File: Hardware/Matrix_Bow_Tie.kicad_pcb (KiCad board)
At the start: 2 copper layers, 116.8 x 55.9 mm, 81 parts, among them J1 CONN_12, J2 CONN_12, Q1 TRANS_NPN_DUAL-MBT3904DW1T1, Q2 TRANS_NPN_DUAL-MBT3904DW1T1, Q3 TRANS_NPN_DUAL-MBT3904DW1T1, Q4 TRANS_NPN_DUAL-MBT3904DW1T1, U1 MAX4466, U2 74HC4051-SOIC16

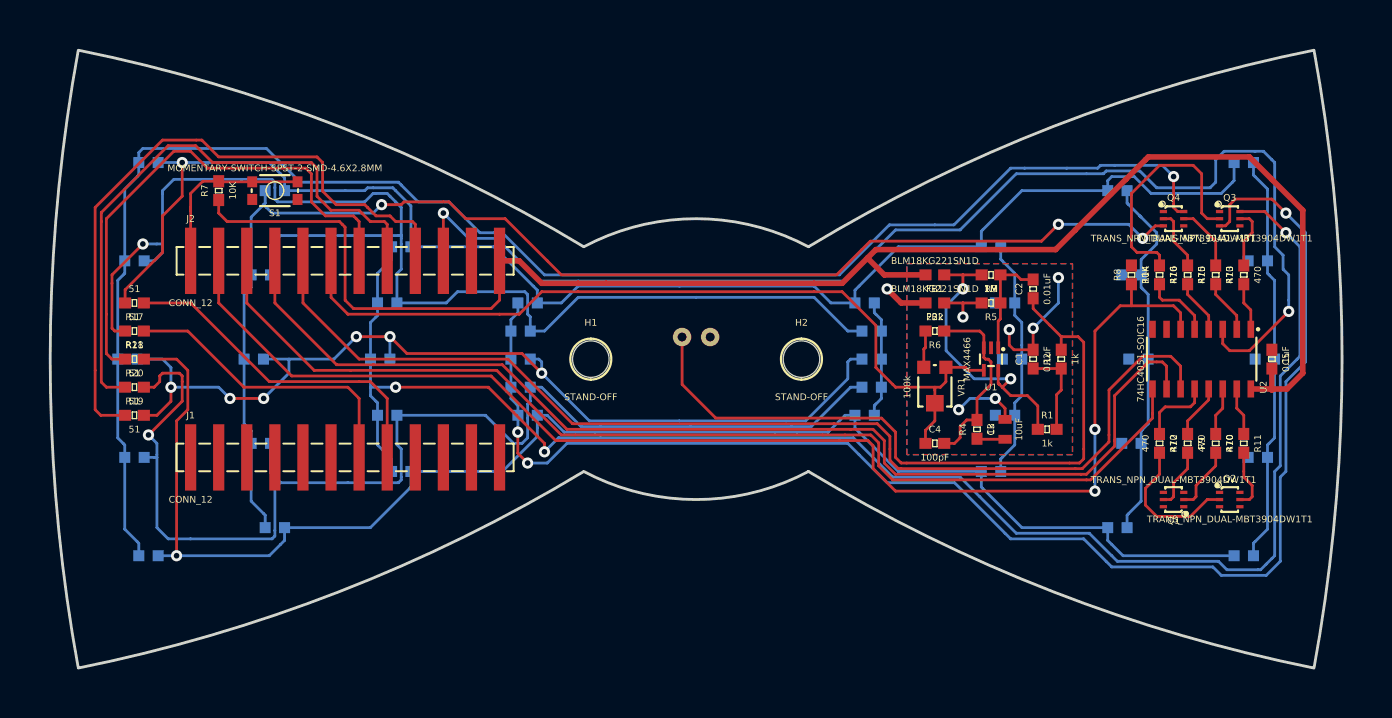
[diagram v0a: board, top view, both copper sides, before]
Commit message: Layout complete. Gerbers ran.
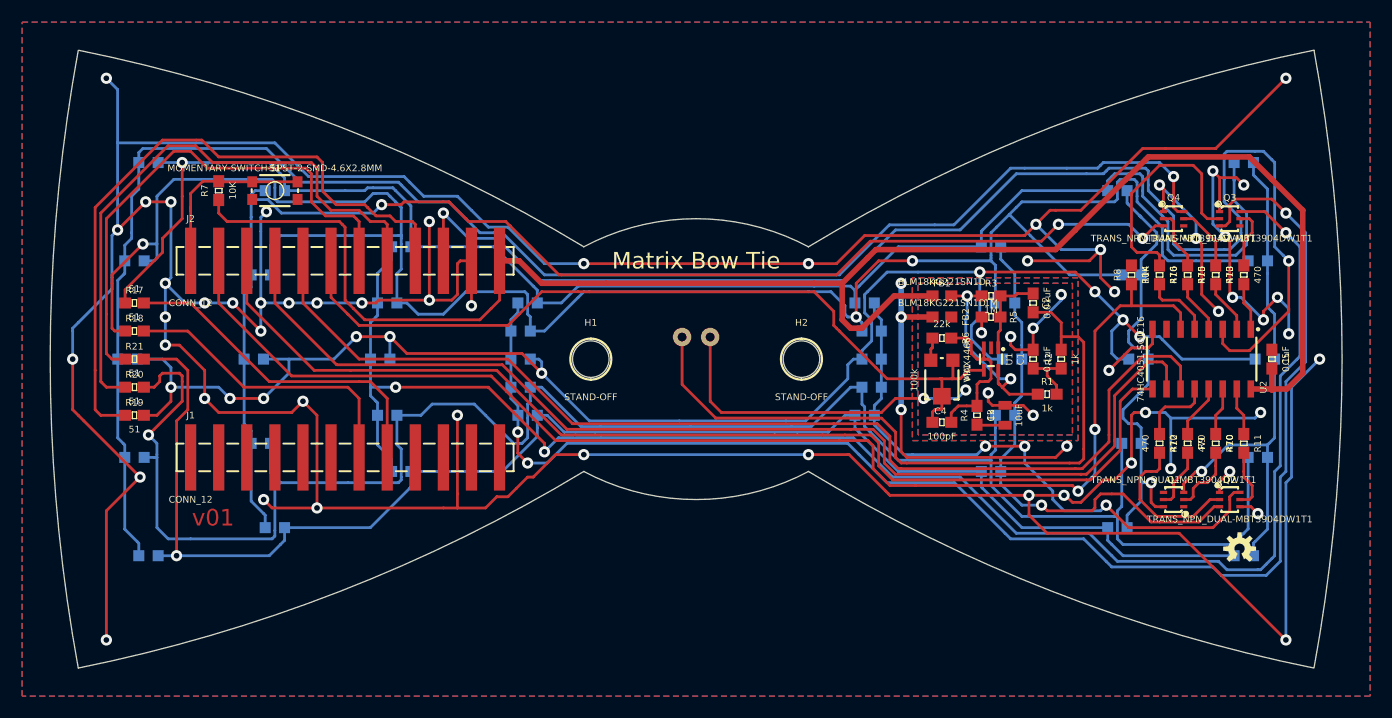
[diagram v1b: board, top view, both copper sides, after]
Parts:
- added LOGO1: OSHW-LOGOS, OSHW-LOGO-S, F.Cu at (209.1, 137.1)
- moved R1 3.17 mm to (191.8, 123.2)
- moved C4 2.01 mm to (182.2, 125.7)
- moved FB1 2.01 mm to (182.2, 114.3)
- moved R3 1.91 mm to (186.7, 114.3)
- moved FB2 1.42 mm to (182.2, 116.2)
- moved C2 1.27 mm to (190.5, 114.9)
- moved C3 1.27 mm to (187.9, 125.1)
- moved R4 1.27 mm to (185.4, 125.1)
- moved R5 1.27 mm to (186.7, 116.2)
- moved R6 0.90 mm to (182.2, 118.1)
- moved VR1 0.90 mm to (182.2, 121.9)
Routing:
- net GND: track 4.07 -> 551.7 mm, vias 1 -> 60
- net Net-(D12-PadA): track 115.9 -> 184.3 mm, vias 1 -> 3
- net Net-(D14-PadA): track 108.7 -> 173.0 mm
- net Net-(D13-PadA): track 88.2 -> 149.2 mm, vias 6 -> 10
- net Net-(D16-PadC): track 10.7 -> 52.9 mm, vias 0 -> 3
- net Net-(D11-PadC): track 21.9 -> 46.5 mm, vias 0 -> 1
- net AGND: track 21.8 -> 46.0 mm, vias 6 -> 8
- net Z: track 112.8 -> 125.5 mm
- net Net-(D1-PadA): track 131.9 -> 143.9 mm
- net Net-(D1-PadC): track 37.1 -> 46.9 mm, vias 0 -> 1
- net 3.3V: track 146.1 -> 154.0 mm
- net VCCA: track 26.7 -> 19.0 mm
- net Net-(D10-PadC): track 33.4 -> 40.7 mm, vias 0 -> 1
- net Net-(C1-Pad1): track 8.22 -> 5.22 mm
- net Net-(C4-Pad2): track 16.8 -> 14.6 mm
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- added copper zone on B.Cu, net GND
- added copper zone on F.Cu, net GND
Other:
- outline, holes or cut-outs redrawn
- board text added: "Matrix Bow Tie"
- board text added: "v01"
